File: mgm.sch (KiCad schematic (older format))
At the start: 26 parts, among them J6 0826-1X1T-GH-F, M1 Fan_4pin, M2 Fan_4pin, U1 rpi_cm4, U4 rpi_cm4

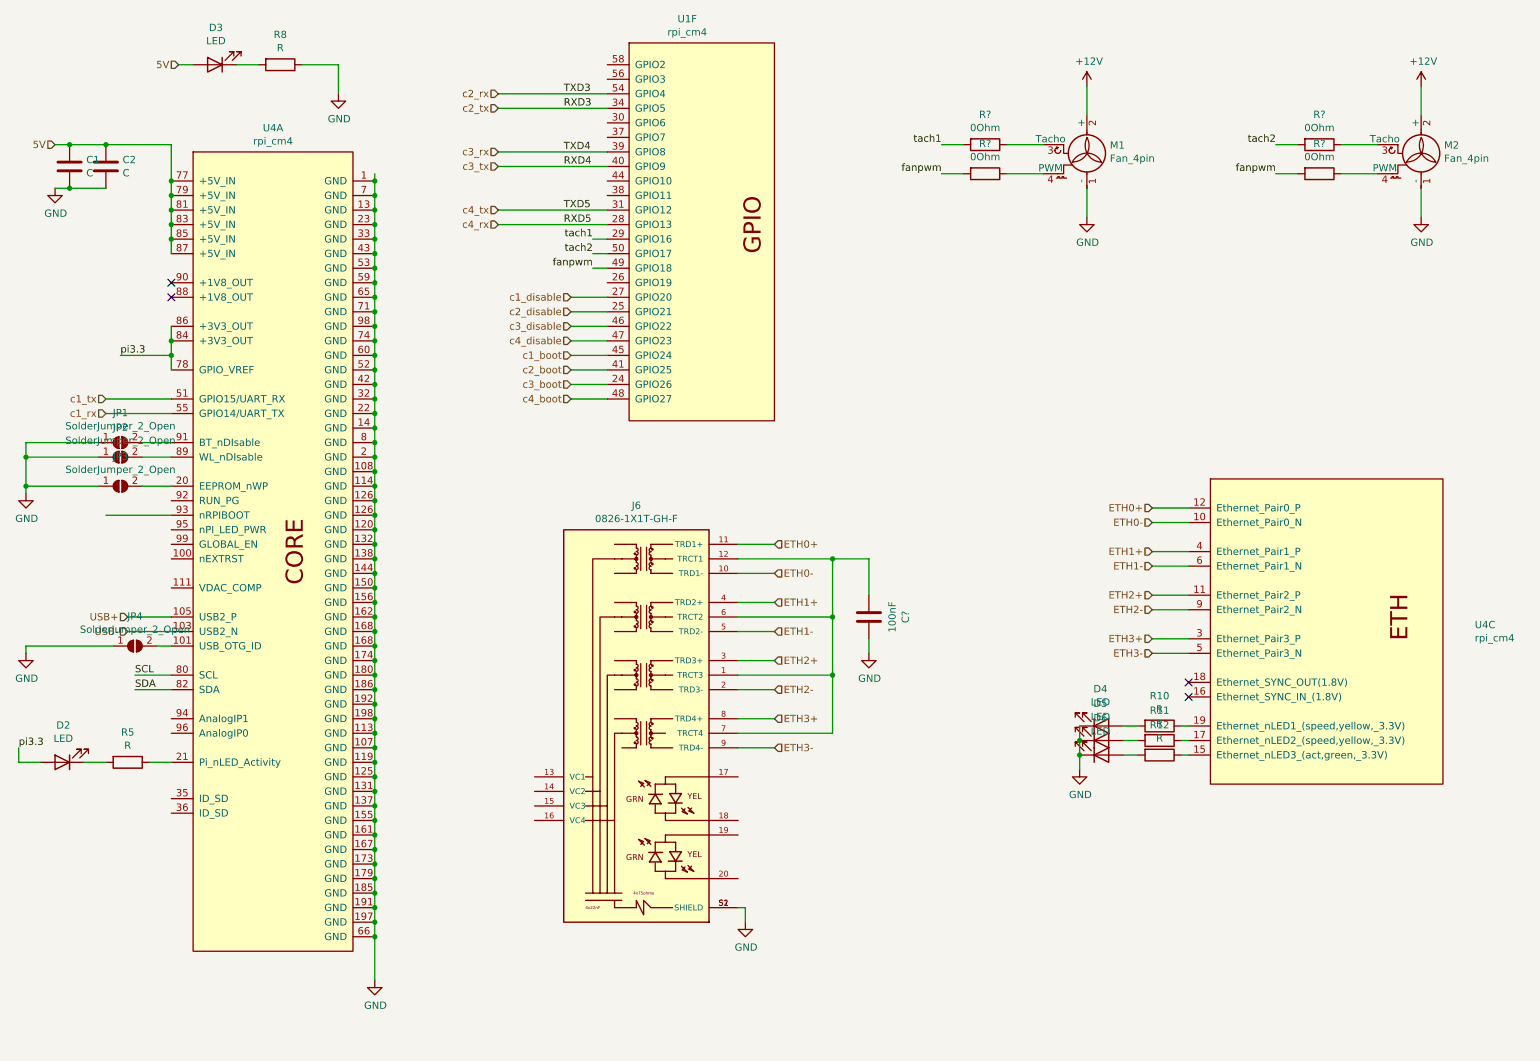
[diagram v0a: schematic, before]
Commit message: Created .gitignore file. Completed schematic organization. Added Fan Driver alternative.
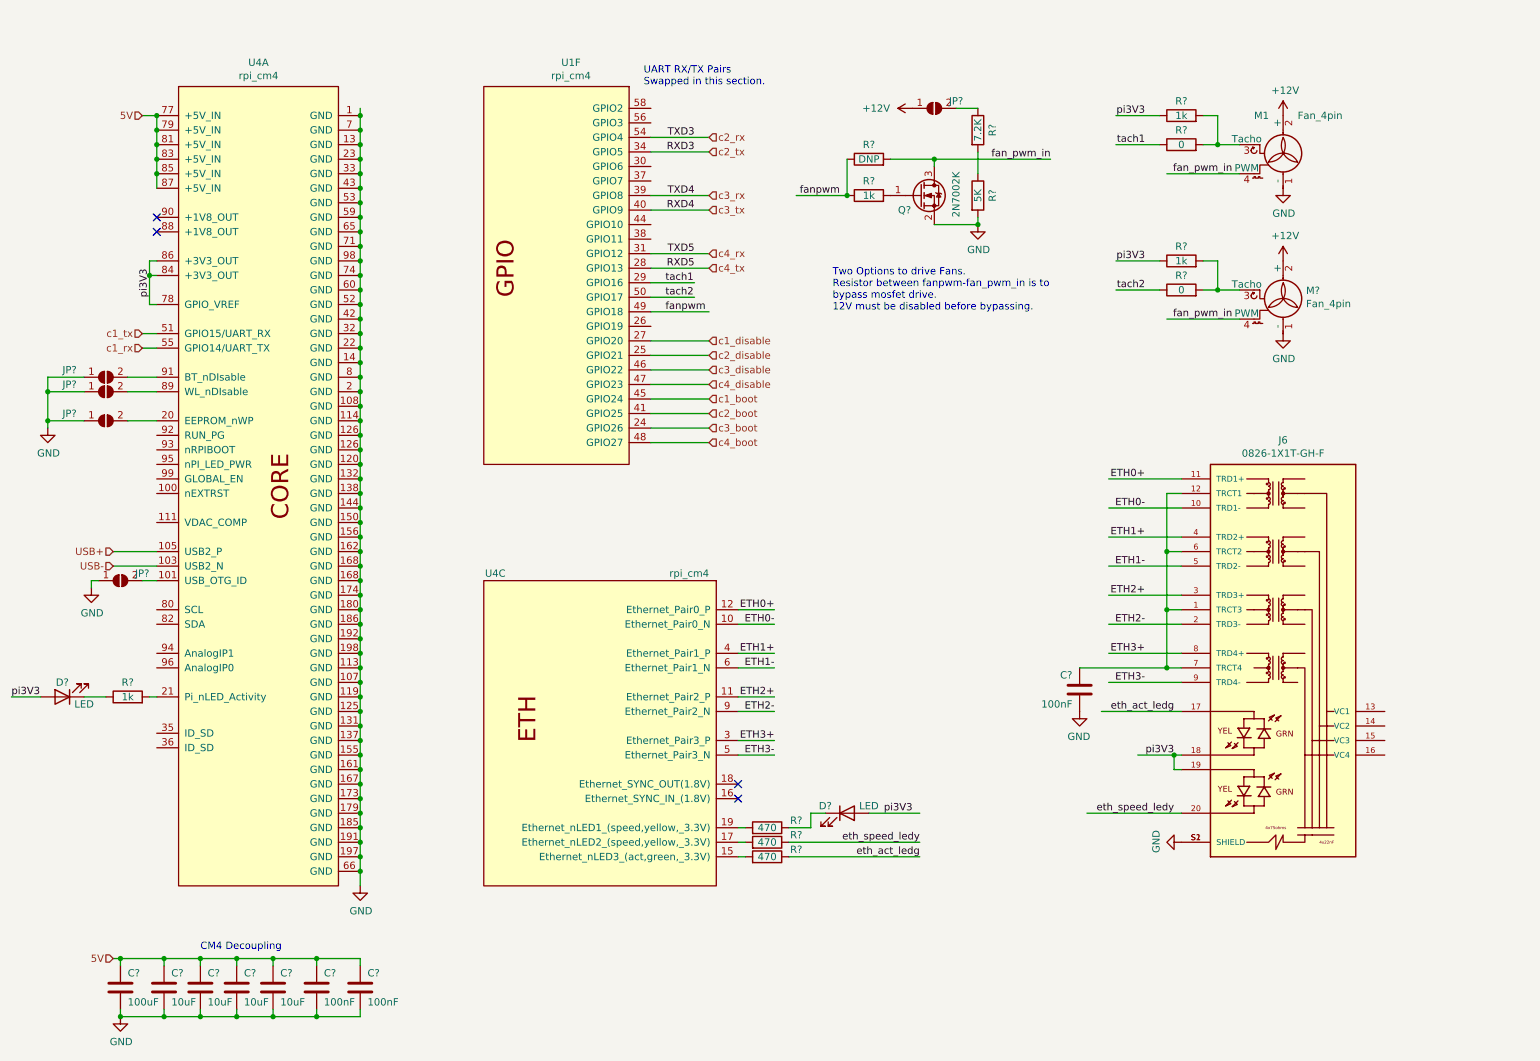
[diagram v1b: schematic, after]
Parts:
- removed C1: C, Capacitor_SMD:C_0805_2012Metric, symbol Device:C
- removed C2: C, Capacitor_SMD:C_0603_1608Metric, symbol Device:C
- removed C?: 100nF, Capacitor_SMD:C_0402_1005Metric, symbol Device:C
- removed D2, D3, D4, D5, D6: LED, LED_SMD:LED_0603_1608Metric, symbol Device:LED
- removed JP1, JP2, JP3, JP4: SolderJumper_2_Open, Jumper:SolderJumper-2_P1.3mm_Open_RoundedPad1.0x1.5mm, symbol Jumper:SolderJumper_2_Open
- removed M2: Fan_4pin, Connector:FanPinHeader_1x04_P2.54mm_Vertical, symbol Motor:Fan_4pin
- removed R10, R11, R12, R5: R, Resistor_SMD:R_0603_1608Metric, symbol Device:R
- removed R8: R, Resistor_SMD:R_0402_1005Metric, symbol Device:R
- removed R? (x4): 0Ohm, Resistor_SMD:R_0402_1005Metric, symbol Device:R
- added C? (x4): 10uF, Capacitor_SMD:C_0805_2012Metric, symbol Device:C
- added C?: 100uF, Capacitor_SMD:C_1206_3216Metric, symbol Device:C
- added C? (x3): 100nF, Capacitor_SMD:C_0402_1005Metric, symbol Device:C
- added D? (x2): LED, LED_SMD:LED_0603_1608Metric, symbol Device:LED
- added JP? (x5): SolderJumper_2_Open, Jumper:SolderJumper-2_P1.3mm_Open_RoundedPad1.0x1.5mm, symbol Jumper:SolderJumper_2_Open
- added M?: Fan_4pin, Connector:FanPinHeader_1x04_P2.54mm_Vertical, symbol Motor:Fan_4pin
- added Q?: 2N7002K, Package_TO_SOT_SMD:SOT-23, symbol Transistor_FET:2N7002K
- added R? (x4): 1k, Resistor_SMD:R_0402_1005Metric, symbol Device:R
- added R? (x3): 470, Resistor_SMD:R_0402_1005Metric, symbol Device:R
- added R? (x2): 0, Resistor_SMD:R_0402_1005Metric, symbol Device:R
- added R?: 7.2K, Resistor_SMD:R_0402_1005Metric, symbol Device:R
- added R?: 5K, Resistor_SMD:R_0402_1005Metric, symbol Device:R
- added R?: DNP, Resistor_SMD:R_0402_1005Metric, symbol Device:R
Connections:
- net labels added: eth_act_ledg, eth_speed_ledy, fan_pwm_in, pi3V3
- net labels removed: SCL, SDA, pi3.3
- wire segments 162 -> 190
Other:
- note added: "CM4 Decoupling"
- note added: "Two Options to drive Fans.\nResistor between fanpwm-fan_pwm_in is to \nbypass mosfet drive. \n12V must be disabled before bypassing."
- note added: "UART RX/TX Pairs \nSwapped in this section."
- moved on the sheet: J6, M1, U1F, U4A, U4C
